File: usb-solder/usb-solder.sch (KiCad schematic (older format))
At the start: 301 parts, among them J1 USB_B_Micro, J10 USB_B_Micro, J11 USB_B_Micro, J12 USB_B_Micro, J13 USB_B_Micro, J14 USB_B_Micro, J15 USB_B_Micro, J16 USB_B_Micro, J17 USB_B_Micro, J18 USB_B_Micro, J19 USB_B_Micro, J2 USB_B_Micro, J20 USB_B_Micro, J21 USB_B_Micro, J22 USB_B_Micro, J23 USB_A, J24 Conn_01x02_Male, J25 Barrel_Jack_Switch, J26 USB_B_Micro, J27 Conn_01x07_Male, J3 USB_B_Micro, J4 USB_B_Micro, J5 USB_B_Micro, J6 USB_B_Micro, J7 USB_B_Micro, J8 USB_B_Micro, J9 USB_B_Micro, SW1 SW_SPDT, U1 555, U2 74HC164, U3 4072, U4 74HC04, U5 AP1117-33

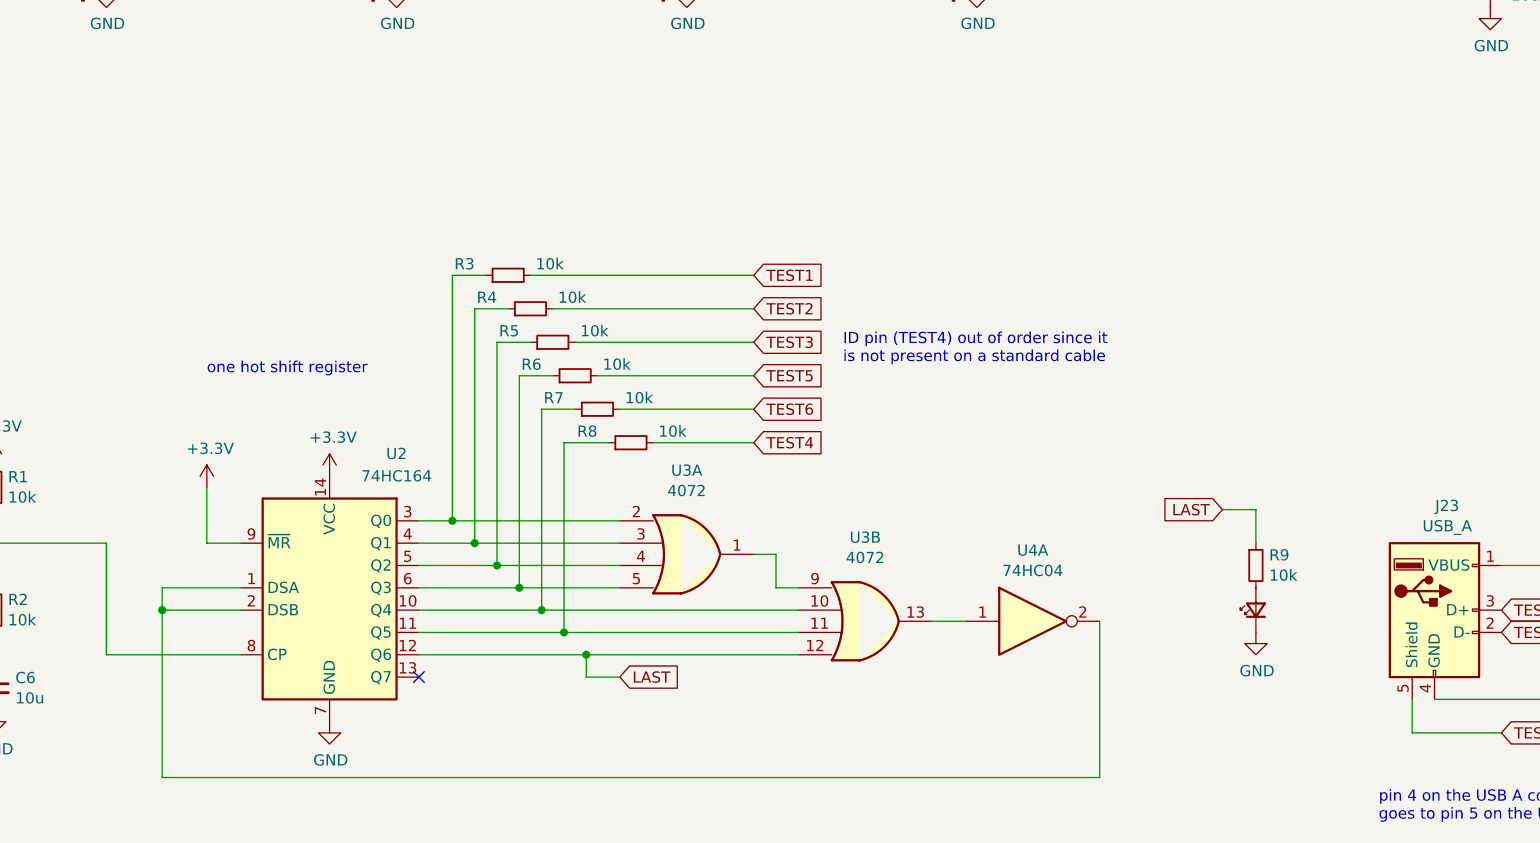
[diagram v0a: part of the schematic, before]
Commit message: routing
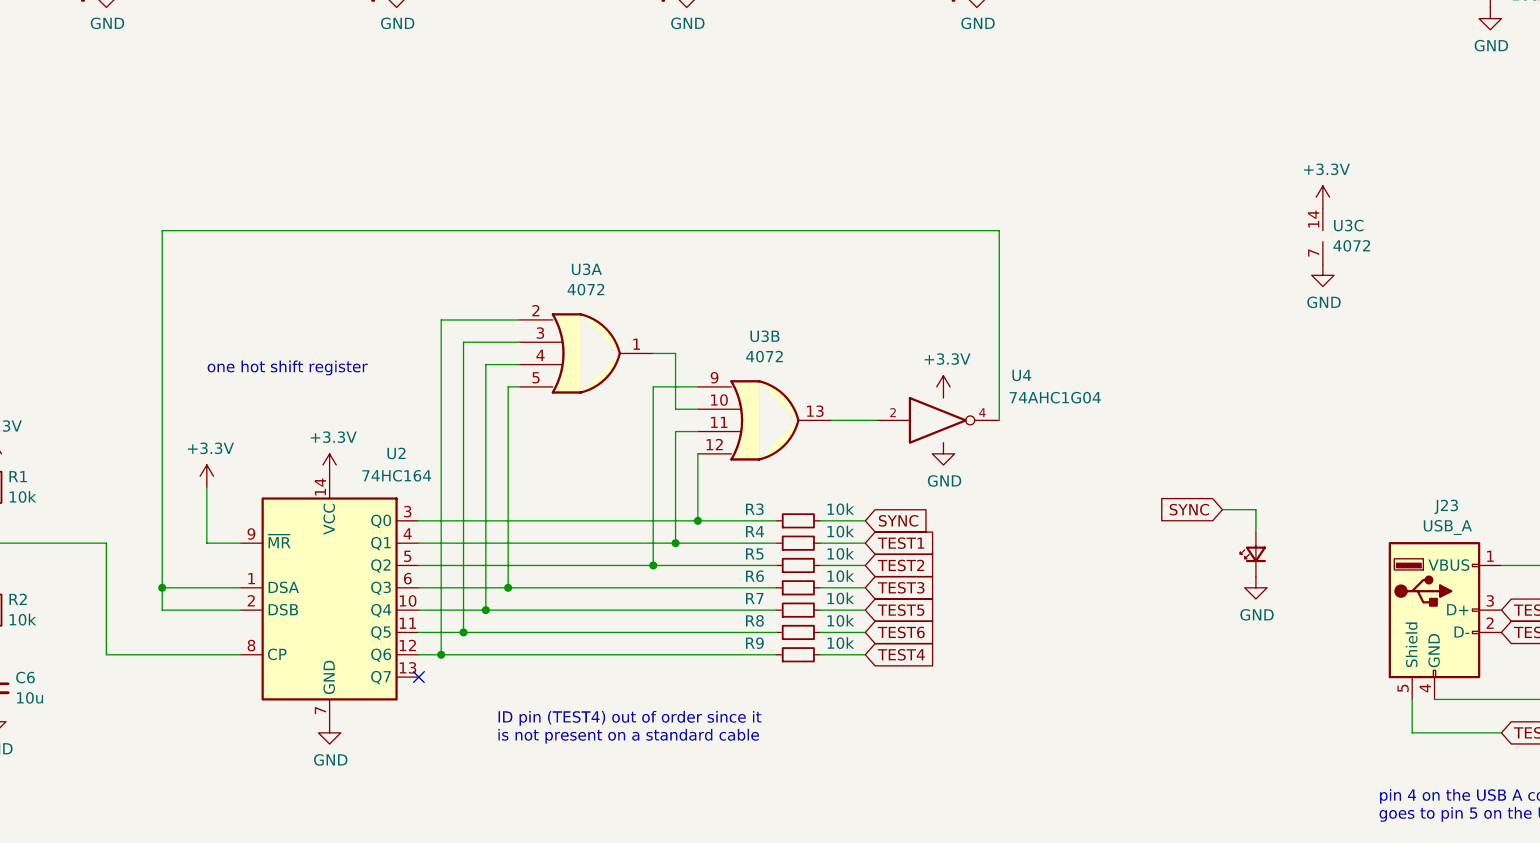
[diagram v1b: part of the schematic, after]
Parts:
- removed U4: 74HC04, Package_SO:SOIC-14_3.9x8.7mm_P1.27mm, symbol pace:74HC04
- added unit 3 of U3
- added U4: 74AHC1G04, Package_TO_SOT_SMD:SOT-353_SC-70-5, symbol pace:74AHC1G04
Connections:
- net +3V3: now also U3.14, U4.5 (VCC)
- net GND: now also U3.7, U4.3 (GND)
- net TEST1: now also R4.2; no longer R3.2
- net TEST2: now also R5.2; no longer R4.2
- net TEST3: now also R6.2; no longer R5.2
- net TEST4: now also R9.2; no longer R8.2
- net TEST5: now also R7.2; no longer R6.2
- net TEST6: now also R8.2; no longer R7.2
- net at U3.13: now also U4.2
- net at U2.1 (DSA), U2.2 (DSB): now also U4.4
- net at R7.1, U2.10 (Q4): now also U3.4; no longer U3.10
- net at R8.1, U2.11 (Q5): now also U3.3; no longer U3.11
- net at R3.1, U2.3 (Q0): now also U3.12; no longer U3.2
- net at R4.1, U2.4 (Q1): now also U3.11; no longer U3.3
- net at R5.1, U2.5 (Q2): now also U3.9; no longer U3.4
- net at U3.1: now also U3.10; no longer U3.9
- net SYNC: now reaches D111.2 (A)
- net SYNC: now also R3.2; no longer R9.2
- net LAST: no longer names the net of R9.1, U2.12 (Q6)
- net LAST: now also U3.2; no longer U3.12
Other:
- moved on the sheet: R3, R4, R5, R6, R7, R8, U3A, U3B
